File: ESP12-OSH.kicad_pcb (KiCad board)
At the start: 2 copper layers, 46.1 x 38.2 mm, 23 parts, among them P1 CONN_01X02, P2 CONN_01X06, P3 CONN_01X08, P4 CONN_01X08, SW1 SW_Push, SW2 SW_Push, U1 ESP-12E

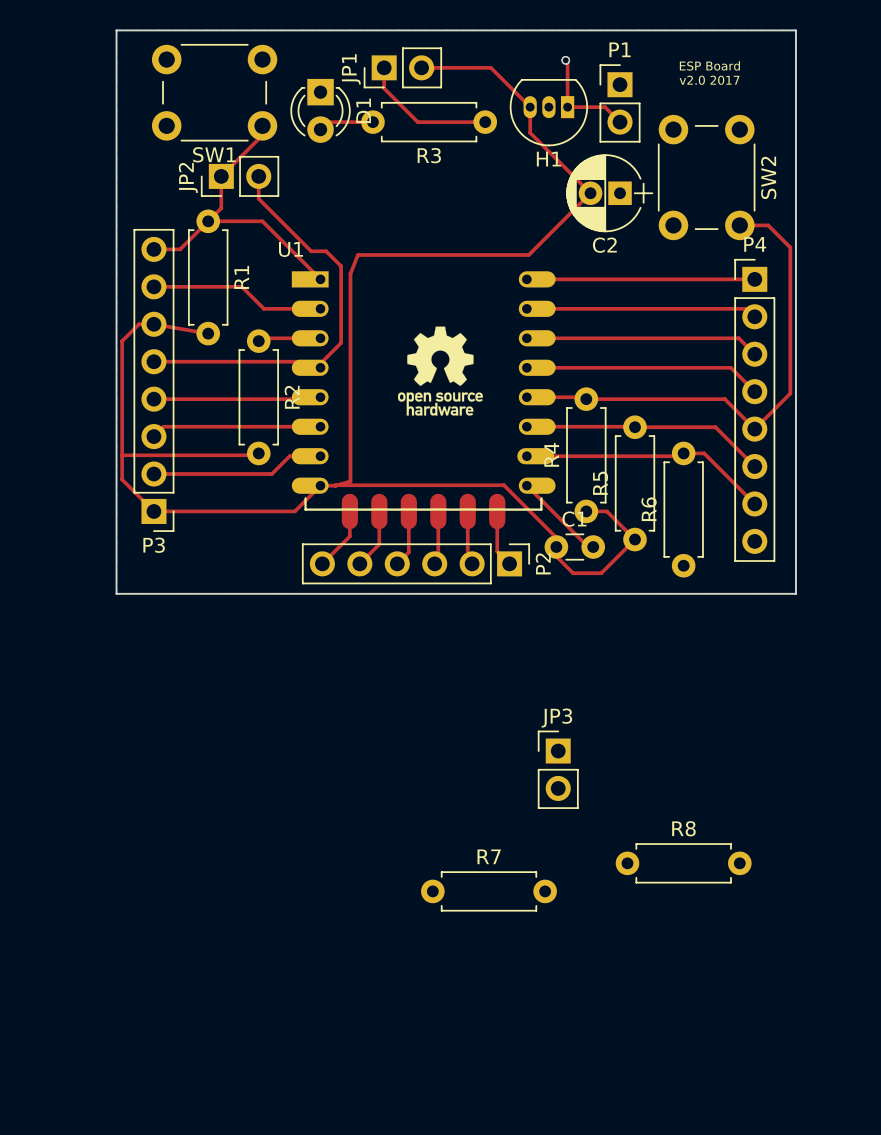
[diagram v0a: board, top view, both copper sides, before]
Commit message: version 2 in the works!
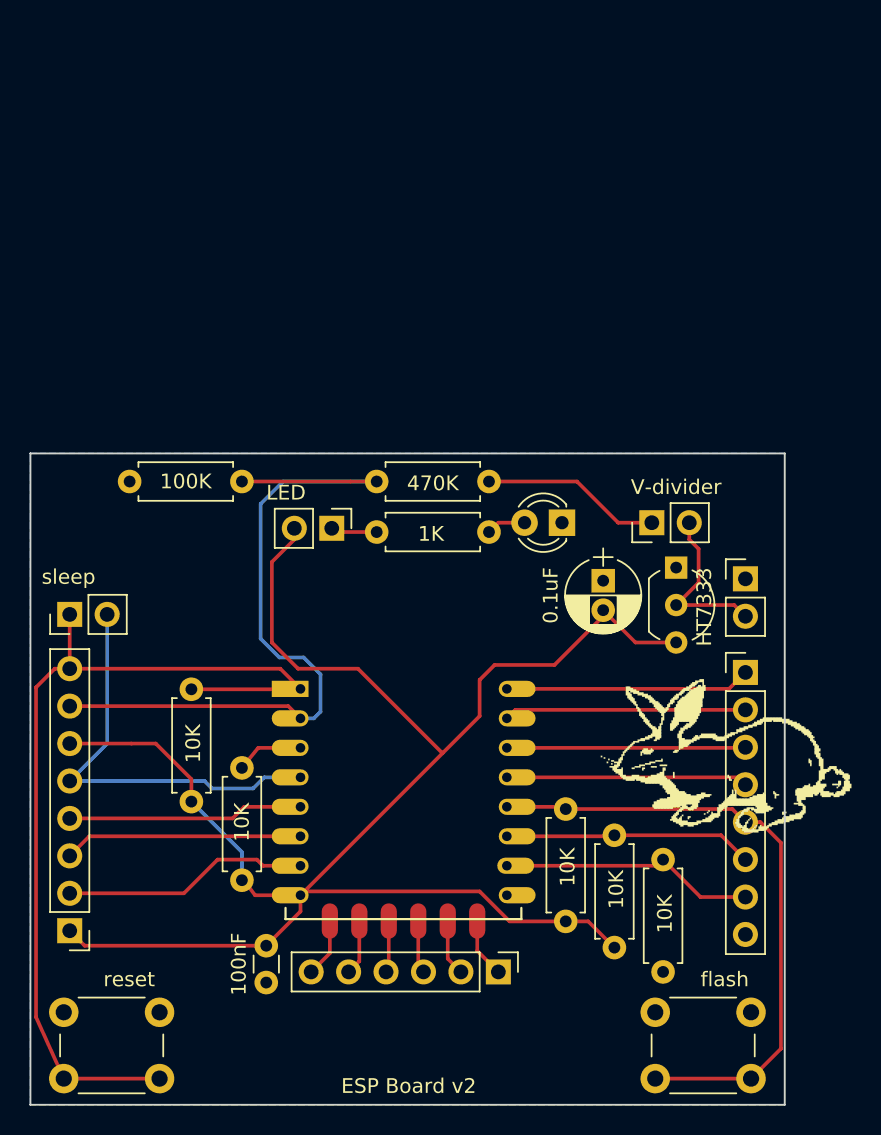
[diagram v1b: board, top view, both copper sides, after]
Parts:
- removed REF***: OSHW-Logo_5.7x6mm_SilkScreen, Symbols:OSHW-Logo_5.7x6mm_SilkScreen
- added LOGO: , ESP12:newlogo, F.Cu at (168.3, 104.1)
- H1: footprint TO_SOT_Packages_THT:TO-92_Inline_Narrow_Oval -> TO_SOT_Packages_THT:TO-92_Inline_Wide
- moved SW1 65.0 mm to (138.9, 131.4)
- moved SW2 64.4 mm to (179.1, 131.4), turned to 180 degrees
- moved P1 34.6 mm to (178.7, 97.5)
- moved D1 33.5 mm to (166.2, 93.7), turned to 180 degrees
- moved C1 33.5 mm to (146.2, 122.4), turned to 270 degrees
- moved H1 32.1 mm to (174.0, 96.8), turned to 270 degrees
- moved R1 31.8 mm to (141.1, 105.0)
- moved JP2 31.4 mm to (132.8, 99.9)
- moved JP1 31.4 mm to (150.6, 94.1), turned to 270 degrees
- moved R7 30.7 mm to (144.5, 90.9), turned to 180 degrees
- moved P3 29.0 mm to (132.8, 121.4)
- moved R2 29.0 mm to (144.5, 110.4)
- moved R3 28.8 mm to (153.7, 94.4), turned to 0 degrees
- moved R4 27.8 mm to (166.5, 120.8)
- moved U1 27.8 mm to (148.5, 105.0)
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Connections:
- H1 pad 1: /VIN -> GND
- H1 pad 2: GND -> /VIN
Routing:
- net /REST: track 21.7 -> 64.3 mm
- net /ADC: track 11.9 -> 51.9 mm
- net Net-(JP3-Pad1): track 0.00 -> 12.2 mm
- net /GPIO0: track 33.7 -> 43.0 mm
- net GND: track 6.23 -> 0.00 mm
- net Net-(JP1-Pad1): track 9.33 -> 3.15 mm
- net /GPIO13: track 11.8 -> 16.8 mm
- net /GPIO14: track 11.4 -> 16.0 mm
- net /GPIO12: track 11.6 -> 16.2 mm
- net /VIN: track 7.33 -> 11.5 mm, vias 1 -> 0
- net /TX: track 15.5 -> 16.7 mm
- net /MOSI: track 3.68 -> 4.86 mm
- net /VCC: track 121.2 -> 122.3 mm
- net Net-(D1-Pad2): track 3.77 -> 2.68 mm
- net /RX: track 15.7 -> 16.4 mm
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- added copper zone on B.Cu, net GND
- removed copper zone on B.Cu, net /GND
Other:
- board size 46.1 x 38.2 mm -> 51.2 x 44.2 mm
- board text added: "ESP Board v2"
- board text added: "LED"
- board text added: "V-divider"
- board text added: "flash"
- board text added: "reset"
- board text added: "sleep"
- board text removed: "ESP Board v2.0 2017"
